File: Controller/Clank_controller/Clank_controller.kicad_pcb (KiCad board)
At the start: 2 copper layers, 104 x 95 mm, 31 parts, among them J1 Limit_SW, J10 Screw_Terminal_01x02, J11 Screw_Terminal_01x02, J12 +5V Conn, J13 Screw_Terminal_01x02, J14 +5V Conn, J15 +5V Conn, J16 Conn_02x13_Odd_Even, J17 +5V Conn, J18 +5V Conn, J2 Limit_SW, J3 Limit_SW, J4 Limit_SW, J5 Limit_SW, J6 Limit_SW, J7 Conn_02x03_Counter_Clockwise, J8 Conn_02x03_Counter_Clockwise, J9 Conn_02x03_Counter_Clockwise

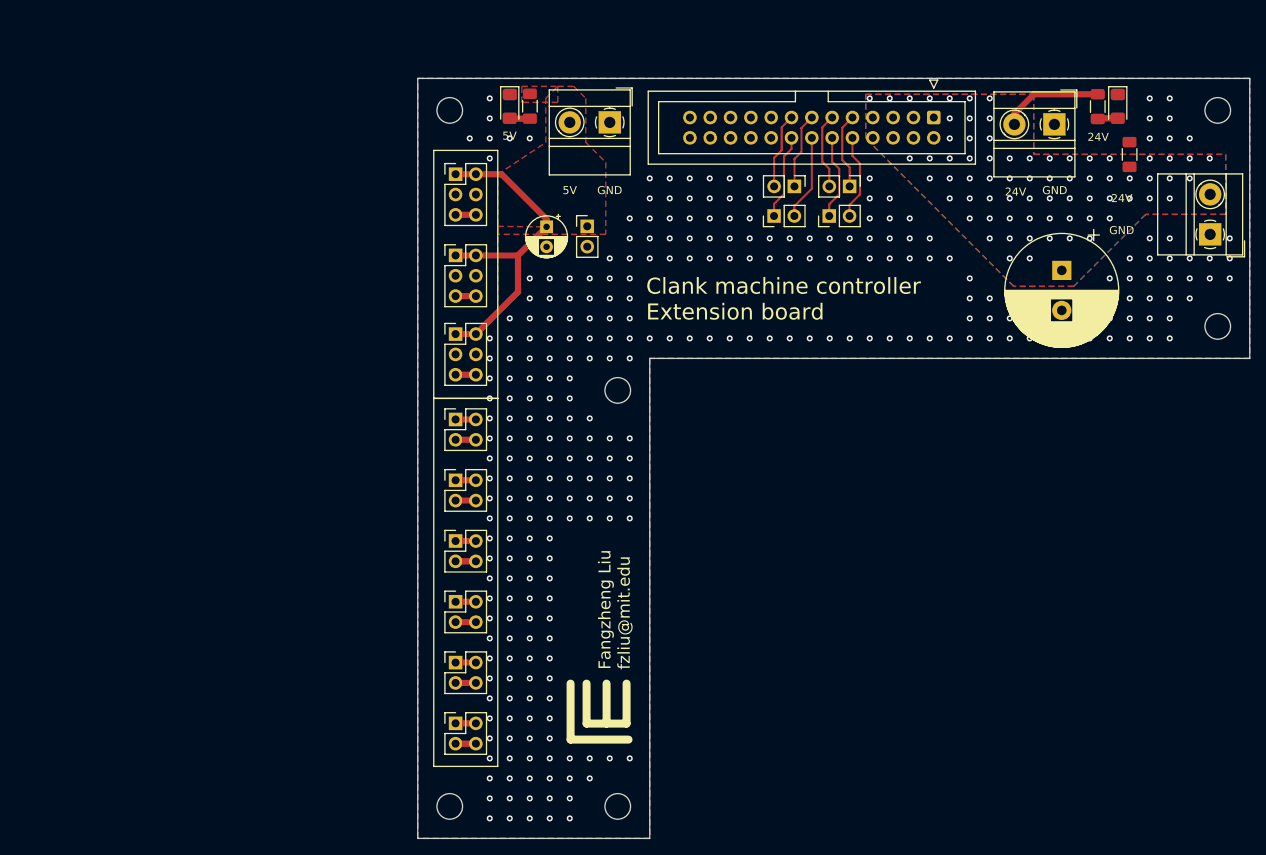
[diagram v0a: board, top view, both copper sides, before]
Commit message: udated by FZ
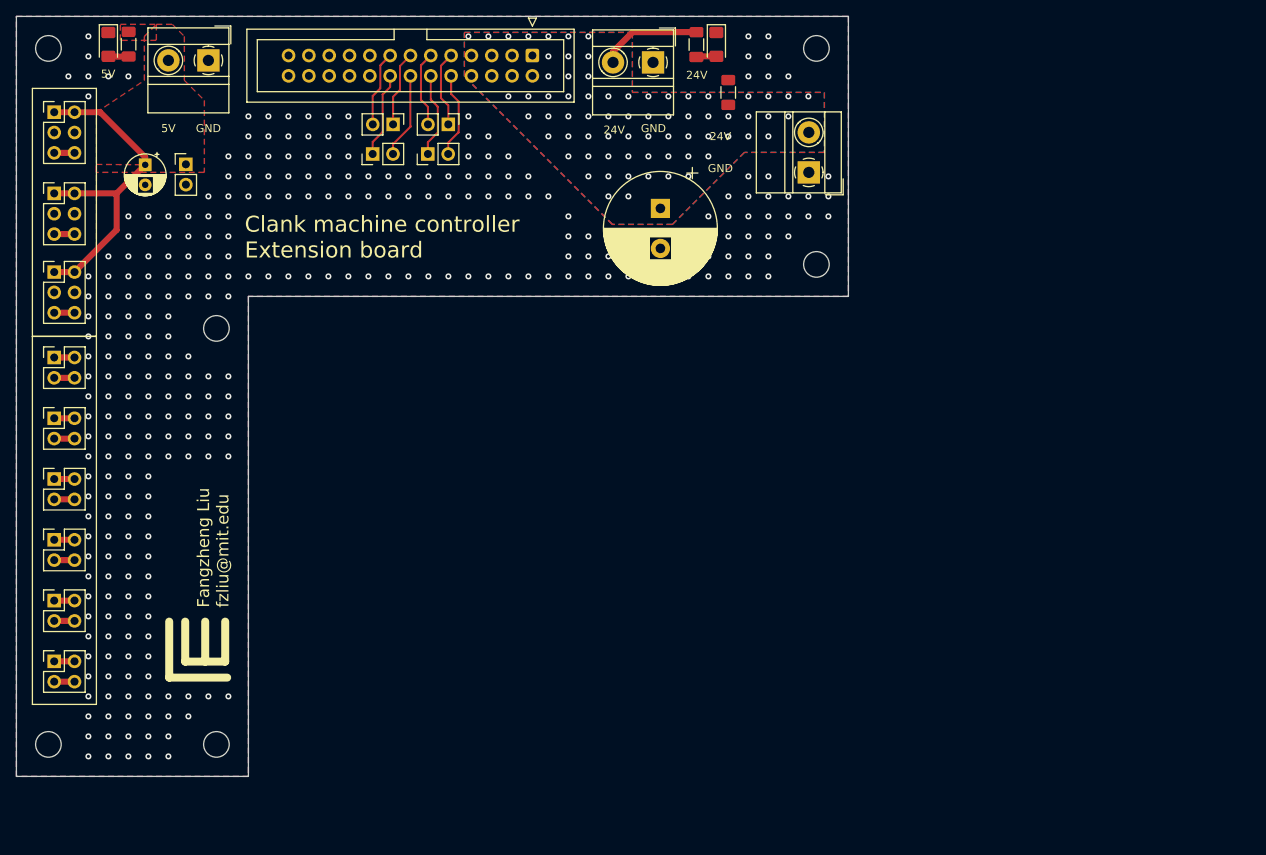
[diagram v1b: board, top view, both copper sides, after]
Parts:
- moved J11 50.8 mm to (175.4, 63.0)
- moved J13 50.8 mm to (194.9, 76.8)
- moved J14 50.8 mm to (149.8, 70.8)
- moved J15 50.8 mm to (142.9, 70.8)
- moved J17 50.8 mm to (147.3, 74.5)
- moved R1 50.8 mm to (109.8, 60.7)
- moved D1 50.8 mm to (107.3, 60.8)
- moved H2 50.8 mm to (99.8, 148.2)
- moved H3 50.8 mm to (99.8, 61.2)
- moved H4 50.8 mm to (120.8, 148.2)
- moved H5 50.8 mm to (120.8, 96.2)
- moved J10 50.8 mm to (119.8, 62.8)
- moved J12 50.8 mm to (117.0, 75.7)
- moved C1 50.8 mm to (111.9, 75.8)
- moved C2 50.8 mm to (176.3, 81.2)
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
